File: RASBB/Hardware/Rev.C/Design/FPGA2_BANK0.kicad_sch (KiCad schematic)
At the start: 18 parts, among them J15 Conn_01x06_Socket, U11 XC7A100T-CSG324

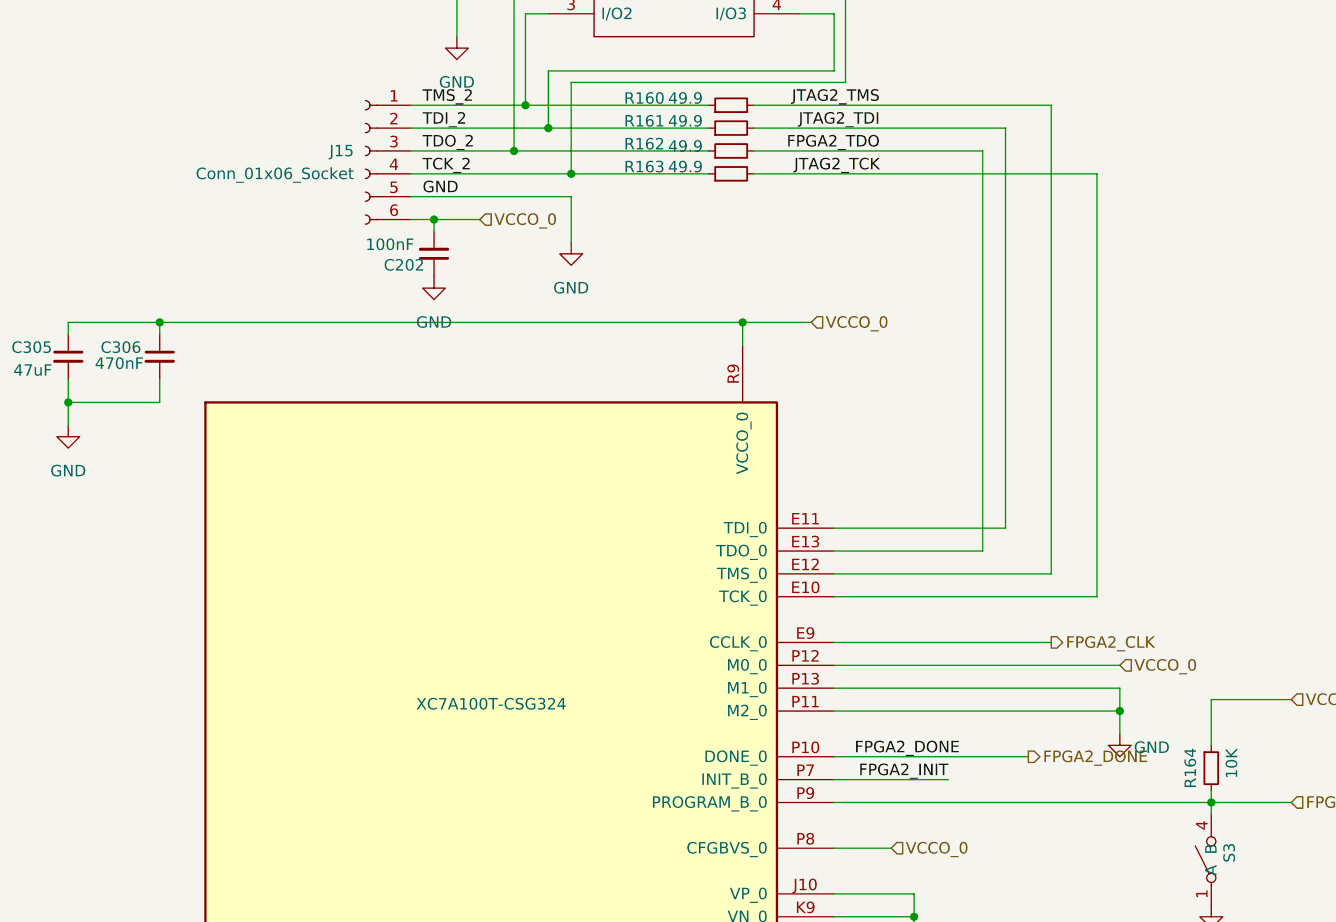
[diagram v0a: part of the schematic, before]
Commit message: RevC_06
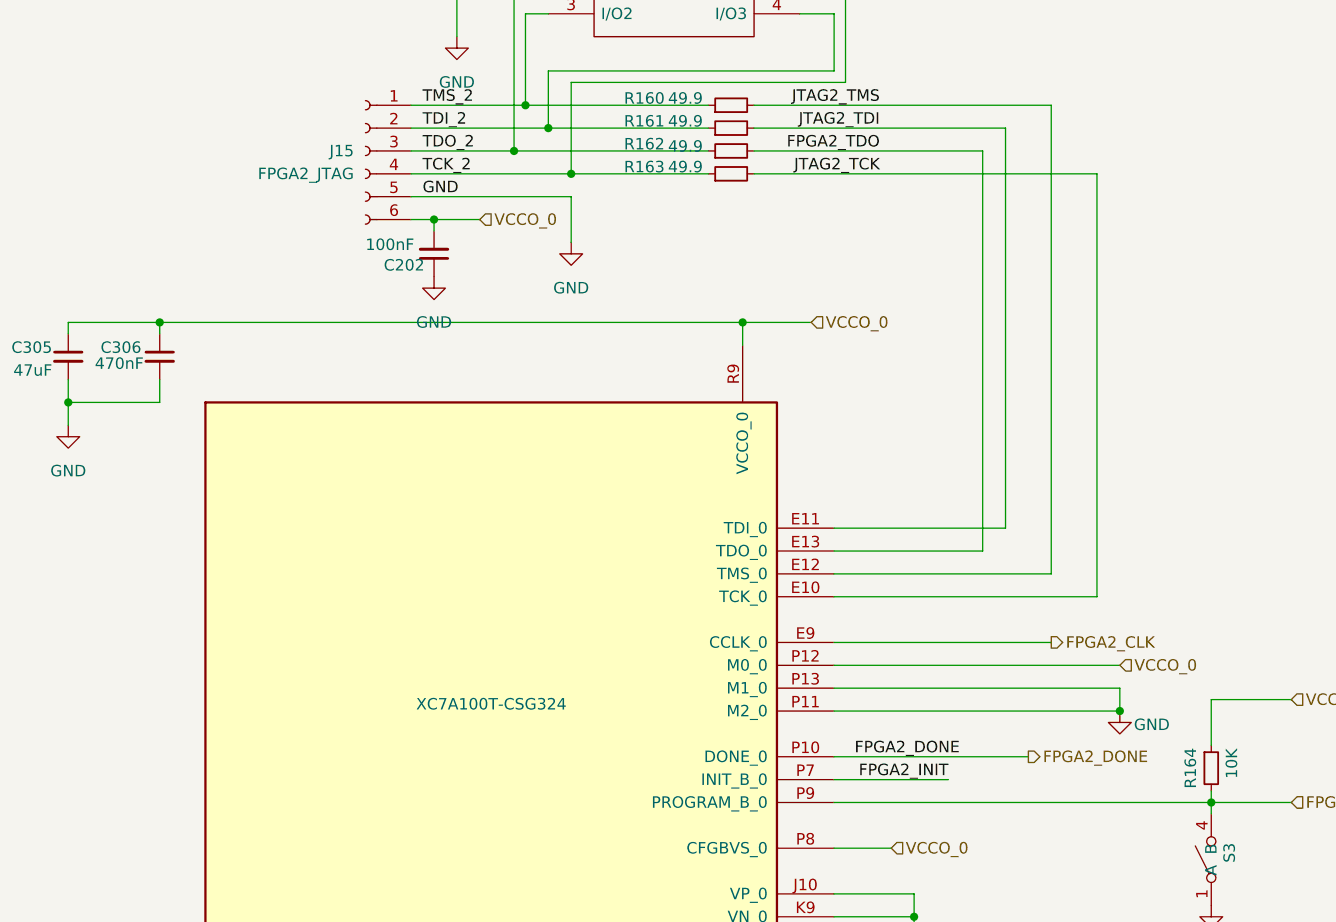
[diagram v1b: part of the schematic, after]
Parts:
- C305: Mfr. Part #  GRM21BR61A476ME15L -> (none)
- C306: Mfr. Part # GRT155R71A474KE01D -> GRM155R71C474KE01D
- D14, D16: LCSC Part #   C5355433 -> (none); Mfr. Part #   A-SP192YR6C-C01-4T -> (none)
- J15: value Conn_01x06_Socket -> FPGA2_JTAG
- R103, R207, R56: LCSC Part # C105871 -> C163826; Mfr. Part # RC0402FR-074K7L -> WR04X4701FTL
- U11: Mfr. Part #  XC7A100T-2CSG324I -> (none)
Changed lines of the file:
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@@
 	(title_block
 		(title "RASBB")
-		(date "2026-09-20")
-		(rev "C")
+		(date "2026-09-27")
+		(rev "C.6")
 		(company "Mina Daneshpajouh")
 	)
@@
 			(width 0)
 			(type default)
+			(color 220 0 0 1)
 		)
 	)
@@
 			(width 0)
 			(type default)
+			(color 220 0 0 1)
 		)
 	)
@@
 			(width 0)
 			(type default)
+			(color 220 0 0 1)
 		)
 	)
@@
 			(width 0)
 			(type default)
+			(color 220 0 0 1)
 		)
 	)
@@
 			(width 0)
 			(type default)
+			(color 220 0 0 1)
 		)
 	)
@@
 			(width 0)
 			(type default)
+			(color 220 0 0 1)
 		)
 	)
@@
 			(width 0)
 			(type default)
+			(color 220 0 0 1)
 		)
 	)
@@
 			(width 0)
 			(type default)
+			(color 220 0 0 1)
 		)
 	)
@@
 			(width 0)
 			(type default)
+			(color 220 0 0 1)
 		)
 	)
@@
 			(width 0)
 			(type default)
+			(color 220 0 0 1)
 		)
 	)
@@
 			(width 0)
 			(type default)
+			(color 220 0 0 1)
 		)
 	)
@@
 			(width 0)
 			(type default)
+			(color 220 0 0 1)
 		)
 	)
@@
 			(width 0)
 			(type default)
-		)
-	)
-	(wire
-		(pts
-			(xy 157.48 109.22) (xy 157.48 111.76)
-		)
-		(stroke
-			(width 0)
-			(type default)
+			(color 220 0 0 1)
 		)
 	)
@@
 			(width 0)
 			(type default)
+			(color 220 0 0 1)
 		)
 	)
@@
 			(width 0)
 			(type default)
+			(color 220 0 0 1)
 		)
 	)
@@
 			(width 0)
 			(type default)
+			(color 220 0 0 1)
 		)
 	)
@@
 			(width 0)
 			(type default)
+			(color 220 0 0 1)
 		)
 	)
@@
 			(width 0)
 			(type default)
+			(color 220 0 0 1)
 		)
 	)
@@
 			(width 0)
 			(type default)
+			(color 220 0 0 1)
 		)
 	)
@@
 			(width 0)
 			(type default)
+			(color 220 0 0 1)
 		)
 	)
@@
 			(width 0)
 			(type default)
+			(color 220 0 0 1)
 		)
 	)
@@
 			)
 		)
-		(property "Mfr. Part #  " "A-SP192YR6C-C01-4T"
-			(at 228.6 130.81 0)
-			(hide yes)
-			(show_name no)
-			(do_not_autoplace no)
-			(effects
-				(font
-					(size 1.27 1.27)
-				)
-			)
-		)
-		(property "LCSC Part #  " "C5355433"
-			(at 228.6 130.81 0)
-			(hide yes)
-			(show_name no)
-			(do_not_autoplace no)
-			(effects
-				(font
-					(size 1.27 1.27)
-				)
-			)
-		)
 		(property "LCSC Part #" "C5355433"
 			(at 228.6 130.81 0)
@@
 			)
 		)
-		(property "Description" "Resistor, small symbol"
+		(property "Description" "62.5mW Thick Film Resistors 50V ±100ppm/℃ ±1% 49.9Ω 0402 Chip Resistor - Surface Mount ROHS"
 			(at 114.3 49.53 0)
 			(hide yes)
@@
 			)
 		)
-		(property "Description" "Resistor, small symbol"
+		(property "Description" "62.5mW Thick Film Resistors 50V ±100ppm/℃ ±1% 49.9Ω 0402 Chip Resistor - Surface Mount ROHS"
 			(at 114.3 44.45 0)
 			(hide yes)
@@
 			)
 		)
-		(property "Mfr. Part #  " "A-SP192YR6C-C01-4T"
-			(at 203.2 120.65 0)
-			(hide yes)
-			(show_name no)
-			(do_not_autoplace no)
-			(effects
-				(font
-					(size 1.27 1.27)
-				)
-			)
-		)
-		(property "LCSC Part #  " "C5355433"
-			(at 203.2 120.65 0)
-			(hide yes)
-			(show_name no)
-			(do_not_autoplace no)
-			(effects
-				(font
-					(size 1.27 1.27)
-				)
-			)
-		)
 		(property "LCSC Part #" "C5355433"
 			(at 203.2 120.65 0)
@@
 			)
 		)
-		(property "Description" "Resistor, small symbol"
+		(property "Description" "62.5mW Thick Film Resistors 50V ±100ppm/℃ ±1% 4.7kΩ 0402 Chip Resistor - Surface Mount ROHS"
 			(at 228.6 120.65 0)
 			(hide yes)
@@
 			)
 		)
-		(property "Mfr. Part #" "RC0402FR-074K7L "
+		(property "Mfr. Part #" "WR04X4701FTL"
 			(at 228.6 120.65 0)
 			(hide yes)
@@
 			)
 		)
-		(property "LCSC Part #" "C105871"
+		(property "LCSC Part #" "C163826"
 			(at 228.6 120.65 0)
 			(hide yes)
@@
 			)
 		)
-		(property "Description" "Resistor, small symbol"
+		(property "Description" "62.5mW Thick Film Resistors 50V ±100ppm/℃ ±1% 49.9Ω 0402 Chip Resistor - Surface Mount ROHS"
 			(at 114.3 46.99 0)
 			(hide yes)
@@
 			)
 		)
-		(property "Mfr. Part # " "XC7A100T-2CSG324I "
-			(at 87.63 109.22 0)
-			(hide yes)
-			(show_name no)
-			(do_not_autoplace no)
-			(effects
-				(font
-					(size 1.27 1.27)
-				)
-			)
-		)
 		(property "LCSC Part #" "C1521791"
 			(at 87.63 109.22 0)
@@
 			)
 		)
-		(property "Mfr. Part #" "GRT155R71A474KE01D "
+		(property "Mfr. Part #" "GRM155R71C474KE01D"
 			(at 50.8 69.85 0)
 			(hide yes)
@@
 			)
 		)
-		(property "Description" "Resistor, small symbol"
+		(property "Description" "62.5mW Thick Film Resistors 50V ±100ppm/℃ ±1% 10kΩ 0402 Chip Resistor - Surface Mount ROHS"
 			(at 167.64 115.57 0)
 			(hide yes)
@@
 			)
 		)
-		(property "Mfr. Part # " "GRM21BR61A476ME15L"
-			(at 40.64 69.85 0)
-			(hide yes)
-			(show_name no)
-			(do_not_autoplace no)
-			(effects
-				(font
-					(size 1.27 1.27)
-				)
-			)
-		)
 		(property "LCSC Part #" "C124129"
 			(at 40.64 69.85 0)
@@
 			)
 		)
-		(property "Description" "Resistor, small symbol"
+		(property "Description" "62.5mW Thick Film Resistors 50V ±100ppm/℃ ±1% 4.7kΩ 0402 Chip Resistor - Surface Mount ROHS"
 			(at 203.2 113.03 0)
 			(hide yes)
@@
 			)
 		)
-		(property "Mfr. Part #" "RC0402FR-074K7L "
+		(property "Mfr. Part #" "WR04X4701FTL"
 			(at 203.2 113.03 0)
 			(hide yes)
@@
 			)
 		)
-		(property "LCSC Part #" "C105871"
+		(property "LCSC Part #" "C163826"
 			(at 203.2 113.03 0)
 			(hide yes)
@@
 			)
 		)
-		(property "Description" "Resistor, small symbol"
+		(property "Description" "62.5mW Thick Film Resistors 50V ±100ppm/℃ ±1% 4.7kΩ 0402 Chip Resistor - Surface Mount ROHS"
 			(at 219.71 120.65 0)
 			(hide yes)
@@
 			)
 		)
-		(property "Mfr. Part #" "RC0402FR-074K7L "
+		(property "Mfr. Part #" "WR04X4701FTL"
 			(at 219.71 120.65 0)
 			(hide yes)
@@
 			)
 		)
-		(property "LCSC Part #" "C105871"
+		(property "LCSC Part #" "C163826"
 			(at 219.71 120.65 0)
 			(hide yes)
@@
 			)
 		)
-		(property "Value" "Conn_01x06_Socket"
+		(property "Value" "FPGA2_JTAG"
 			(at 72.39 49.5299 0)
 			(show_name no)
@@
 			)
 		)
-		(property "Description" "Resistor, small symbol"
+		(property "Description" "62.5mW Thick Film Resistors 50V ±100ppm/℃ ±1% 49.9Ω 0402 Chip Resistor - Surface Mount ROHS"
 			(at 114.3 41.91 0)
 			(hide yes)
@@
 	(symbol
 		(lib_id "power:GND")
-		(at 157.48 111.76 0)
+		(at 157.48 109.22 0)
 		(mirror y)
 		(unit 1)
@@
 		(dnp no)
 		(property "Reference" "#PWR0241"
-			(at 157.48 118.11 0)
+			(at 157.48 115.57 0)
 			(hide yes)
 			(show_name no)
@@
 		)
 		(property "Value" "GND"
-			(at 161.036 113.284 0)
+			(at 161.036 110.744 0)
 			(show_name no)
 			(do_not_autoplace no)
@@
 		)
 		(property "Footprint" ""
-			(at 157.48 111.76 0)
+			(at 157.48 109.22 0)
 			(hide yes)
 			(show_name no)
@@
 		)
 		(property "Datasheet" ""
-			(at 157.48 111.76 0)
+			(at 157.48 109.22 0)
 			(hide yes)
 			(show_name no)
@@
 		)
 		(property "Description" "Power symbol creates a global label with name \"GND\" , ground"
-			(at 157.48 111.76 0)
+			(at 157.48 109.22 0)
 			(hide yes)
 			(show_name no)
